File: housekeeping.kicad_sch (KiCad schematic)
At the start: 3 parts, among them U4 TPS7B8133QDGNRQ1

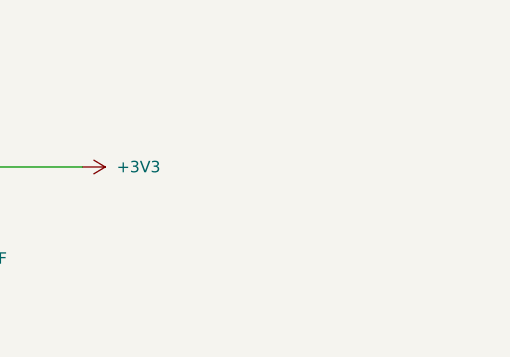
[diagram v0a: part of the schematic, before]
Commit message: Doing placement
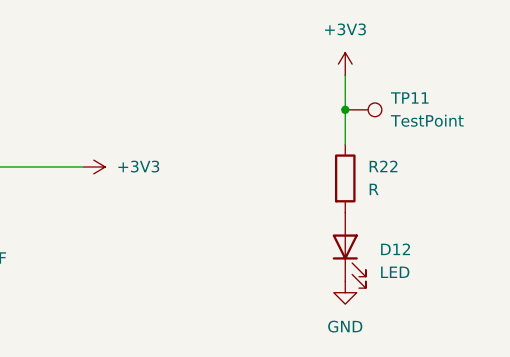
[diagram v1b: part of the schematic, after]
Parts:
- added D12: LED, LED_SMD:LED_0603_1608Metric, symbol Device:LED
- added R22: R, Resistor_SMD:R_0603_1608Metric, symbol Device:R
- added TP11: TestPoint, TestPoint:TestPoint_Pad_D2.0mm, symbol Connector:TestPoint
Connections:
- net +3V3: now also R22.1, TP11.1
- net GND: now also D12.1 (K)
- new net: D12.2 (A), R22.2

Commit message: Prelim placement done
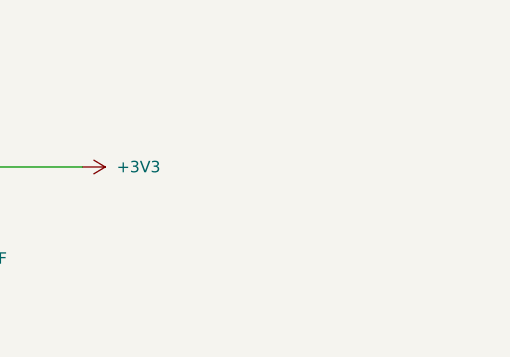
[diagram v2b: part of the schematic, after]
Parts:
- removed D12: LED, LED_SMD:LED_0603_1608Metric, symbol Device:LED
- removed R22: R, Resistor_SMD:R_0603_1608Metric, symbol Device:R
- removed TP11: TestPoint, TestPoint:TestPoint_Pad_D2.0mm, symbol Connector:TestPoint
